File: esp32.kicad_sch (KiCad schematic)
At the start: 38 parts, among them SW2 BOOT, SW3 Reset, U5 ESP32-S3R8, U6 W25Q128JVSIQ, Y1 40MHz

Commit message: rev2 update
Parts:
- L2: Supplier Part C27124 -> C16526
- SW2, SW3: Function (none) -> ESP32; LCSC Part # (none) -> C221897; Manufacturer (none) -> C&K; Manufacturer Part (none) -> PTS810SJS250SMTRLFS; Supplier Part (none) -> C221897
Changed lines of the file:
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@@
 			)
 		)
-		(property "Supplier Part" "C27124"
+		(property "Supplier Part" "C16526"
 			(at 39.37 71.12 90)
 			(effects
@@
 			)
 		)
+		(property "Function" "ESP32"
+			(at 39.37 175.26 90)
+			(effects
+				(font
+					(size 1.27 1.27)
+				)
+				(hide yes)
+			)
+		)
+		(property "Manufacturer" "C&K"
+			(at 39.37 175.26 90)
+			(effects
+				(font
+					(size 1.27 1.27)
+				)
+				(hide yes)
+			)
+		)
+		(property "Manufacturer Part" "PTS810SJS250SMTRLFS"
+			(at 39.37 175.26 90)
+			(effects
+				(font
+					(size 1.27 1.27)
+				)
+				(hide yes)
+			)
+		)
+		(property "Supplier Part" "C221897"
+			(at 39.37 175.26 90)
+			(effects
+				(font
+					(size 1.27 1.27)
+				)
+				(hide yes)
+			)
+		)
+		(property "LCSC Part #" "C221897"
+			(at 39.37 175.26 90)
+			(effects
+				(font
+					(size 1.27 1.27)
+				)
+				(hide yes)
+			)
+		)
 		(pin "1"
 		)
@@
 			(effects
 				(font
+					(size 1.27 1.27)
+				)
+				(hide yes)
+			)
+		)
+		(property "Function" "ESP32"
+			(at 83.82 176.53 90)
+			(effects
+				(font
+					(size 1.27 1.27)
+				)
+				(hide yes)
+			)
+		)
+		(property "Manufacturer" "C&K"
+			(at 83.82 176.53 90)
+			(effects
+				(font
+					(size 1.27 1.27)
+				)
+				(hide yes)
+			)
+		)
+		(property "Manufacturer Part" "PTS810SJS250SMTRLFS"
+			(at 83.82 176.53 90)
+			(effects
+				(font
+					(size 1.27 1.27)
+				)
+				(hide yes)
+			)
+		)
+		(property "Supplier Part" "C221897"
+			(at 83.82 176.53 90)
+			(effects
+				(font
+					(size 1.27 1.27)
+				)
+				(hide yes)
+			)
+		)
+		(property "LCSC Part #" "C221897"
+			(at 83.82 176.53 90)
+			(effects
+				(font

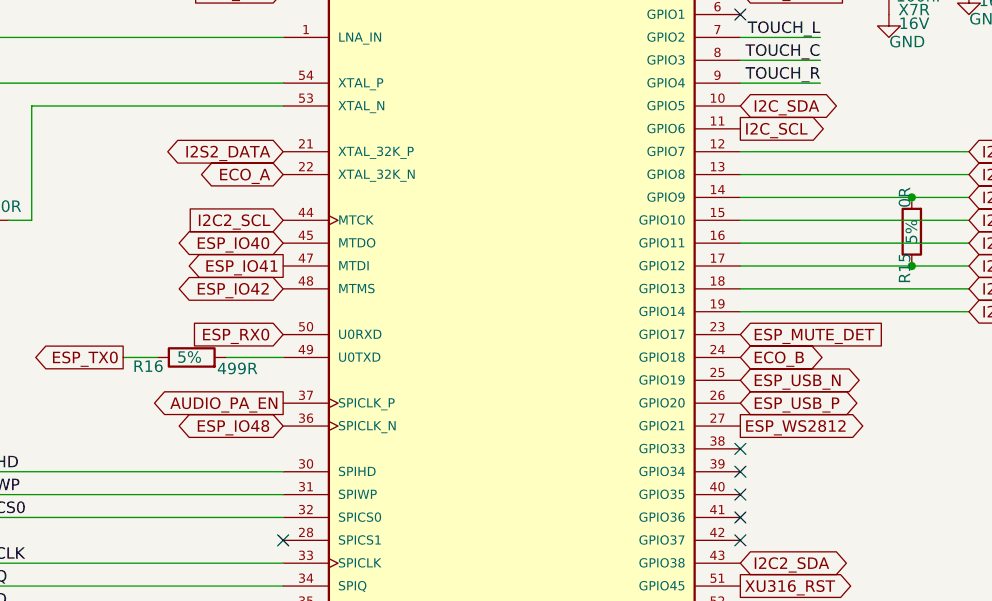
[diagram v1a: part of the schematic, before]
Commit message: update for production
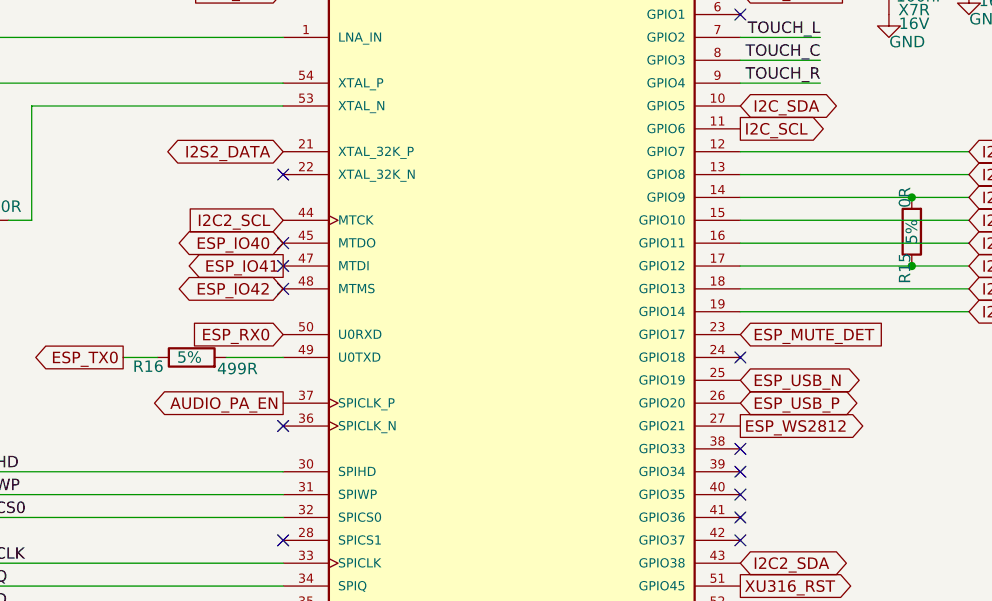
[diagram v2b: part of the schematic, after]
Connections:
- net ECO_A: no longer names the net of U5.22 (XTAL_32K_N)
- net ECO_B: no longer names the net of U5.24 (GPIO18)
- net ESP_IO48: no longer names the net of U5.36 (SPICLK_N)
- no-connect marks 8 -> 14
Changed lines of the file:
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@@
+	)
+	(no_connect
+		(at 162.56 106.68)
+	)
+	(no_connect
+		(at 111.76 86.36)
+	)
+	(no_connect
+		(at 111.76 93.98)
+	)
+	(no_connect
+		(at 111.76 96.52)
 	)
 	(no_connect
@@
 	(no_connect
 		(at 162.56 124.46)
+	)
+	(no_connect
+		(at 111.76 114.3)
+	)
+	(no_connect
+		(at 111.76 99.06)
 	)
 	(no_connect
@@
 		)
 	)
-	(global_label "ECO_A"
-		(shape bidirectional)
-		(at 111.76 86.36 180)
-		(fields_autoplaced yes)
-		(effects
-			(font
-				(size 1.27 1.27)
-			)
-			(justify right)
-		)
-		(property "Intersheetrefs" "${INTERSHEET_REFS}"
-			(at 101.8578 86.36 0)
-			(effects
-				(font
-					(size 1.27 1.27)
-				)
-				(justify right)
-				(hide yes)
-			)
-		)
-	)
 	(global_label "ESP_USB_N"
 		(shape bidirectional)
@@
 				(hide yes)
 			)
-		)
-	)
-	(global_label "ESP_IO48"
-		(shape bidirectional)
-		(at 111.76 114.3 180)
-		(fields_autoplaced yes)
-		(effects
-			(font
-				(size 1.27 1.27)
-			)
-			(justify right)
-		)
-		(property "Intersheetrefs" "${INTERSHEET_REFS}"
-			(at 98.7131 114.3 0)
-			(effects
-				(font
-					(size 1.27 1.27)
-				)
-				(justify right)
-				(hide yes)
-			)
-		)
-	)
-	(global_label "ECO_B"
-		(shape bidirectional)
-		(at 162.56 106.68 0)
-		(fields_autoplaced yes)
-		(effects
-			(font
-				(size 1.27 1.27)
-			)
-			(justify left)
-		)
-		(property "Intersheetrefs" "${INTERSHEET_REFS}"
-			(at 172.6436 106.68 0)
-			(effects
-				(font
-					(size 1.27 1.27)
-				)
-				(justify left)
-				(hide yes)
-			)
